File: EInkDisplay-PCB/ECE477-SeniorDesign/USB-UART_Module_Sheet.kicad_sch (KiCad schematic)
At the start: 8 parts, among them J4 USB_A, U6 NUP2202, U7 CP2102-GMR

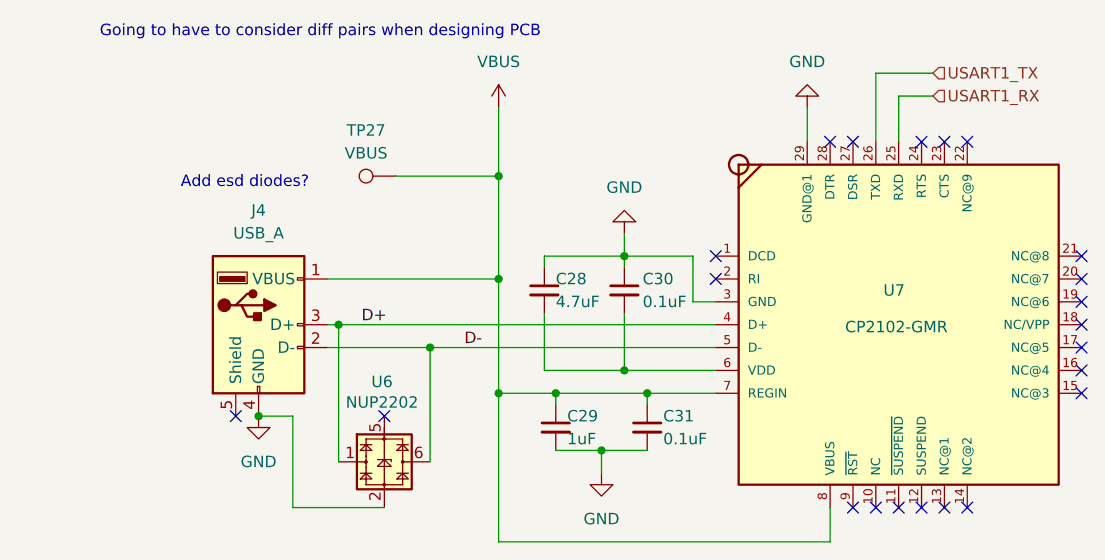
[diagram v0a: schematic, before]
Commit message: pushing
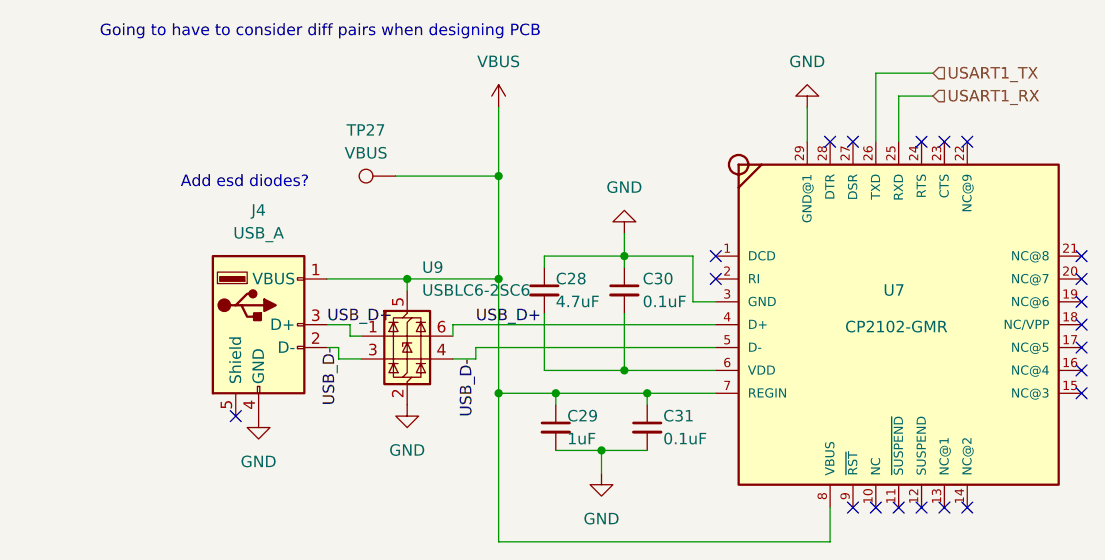
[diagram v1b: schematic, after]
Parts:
- removed U6: NUP2202, Package_TO_SOT_SMD:SOT-363_SC-70-6, symbol Power_Protection:NUP2202
- added U9: USBLC6-2SC6, Package_TO_SOT_SMD:SOT-23-6, symbol Power_Protection:USBLC6-2SC6
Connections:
- net GND: now also U9.2 (GND)
- net VBUS: now also U9.5 (VBUS)
- net D+ renamed USB_D+
- net USB_D+: now also U9.1 (I/O1), U9.6 (I/O1)
- net D- renamed USB_D-
- net USB_D-: now also U9.3 (I/O2), U9.4 (I/O2)
- no-connect marks 22 -> 21
